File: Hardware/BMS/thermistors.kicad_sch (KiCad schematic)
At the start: 6 parts, among them U2 MAX14661ETI+T, U6 MAX14661ETI+T

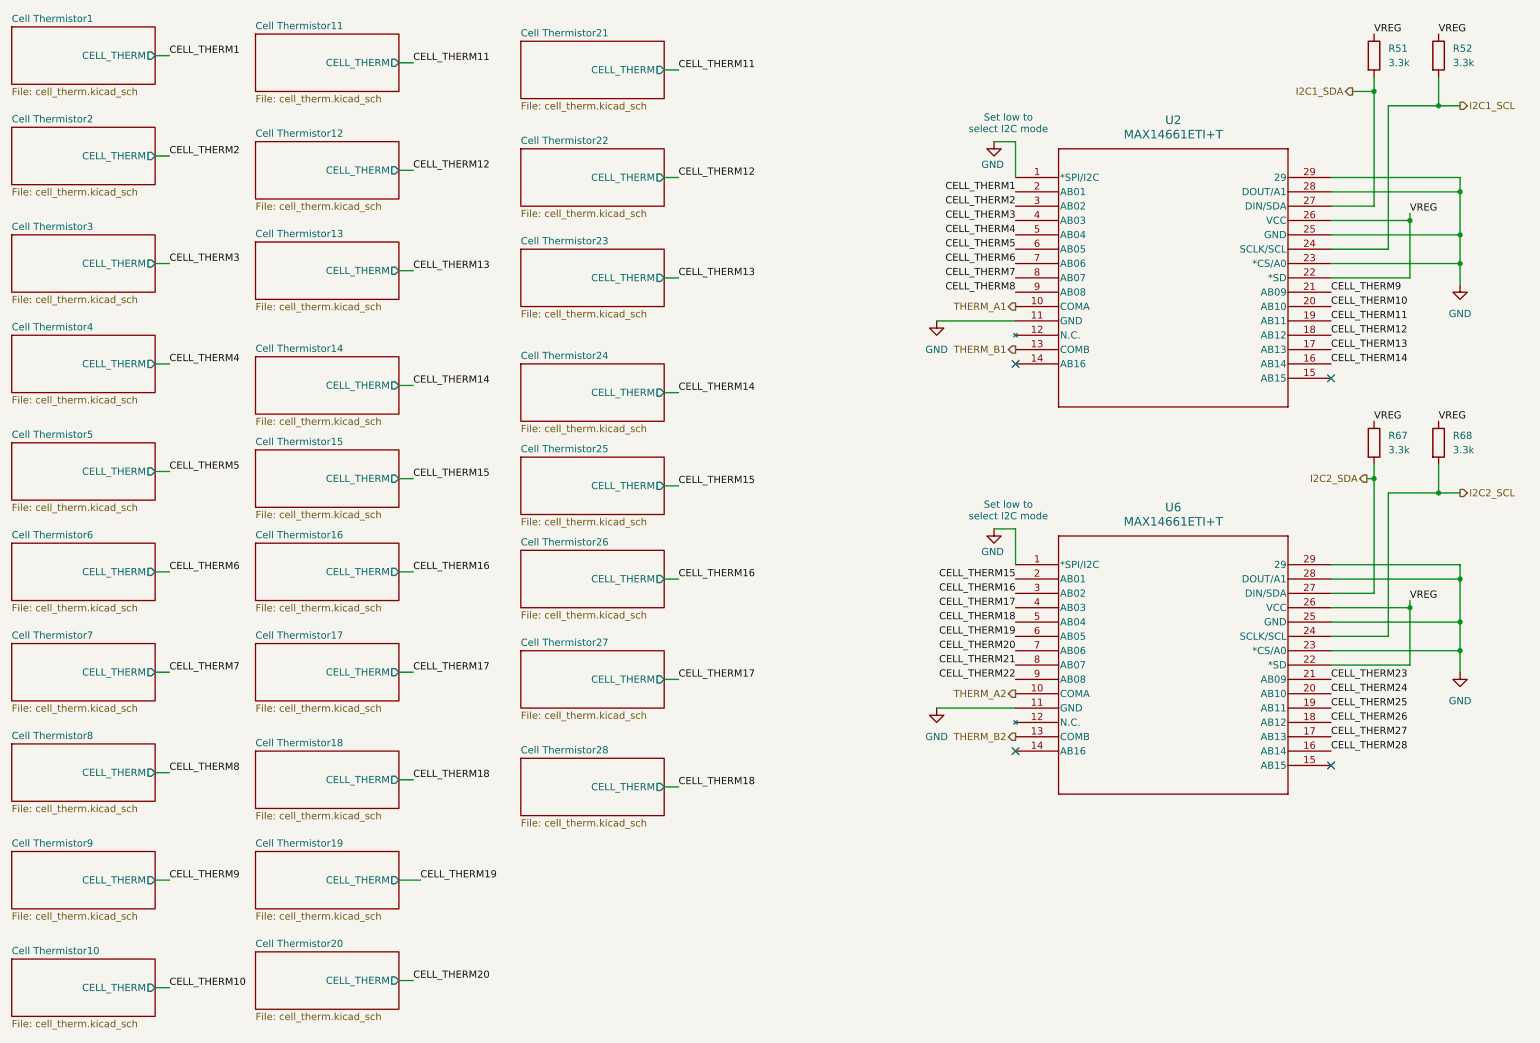
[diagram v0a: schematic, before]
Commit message: edits to the BMS
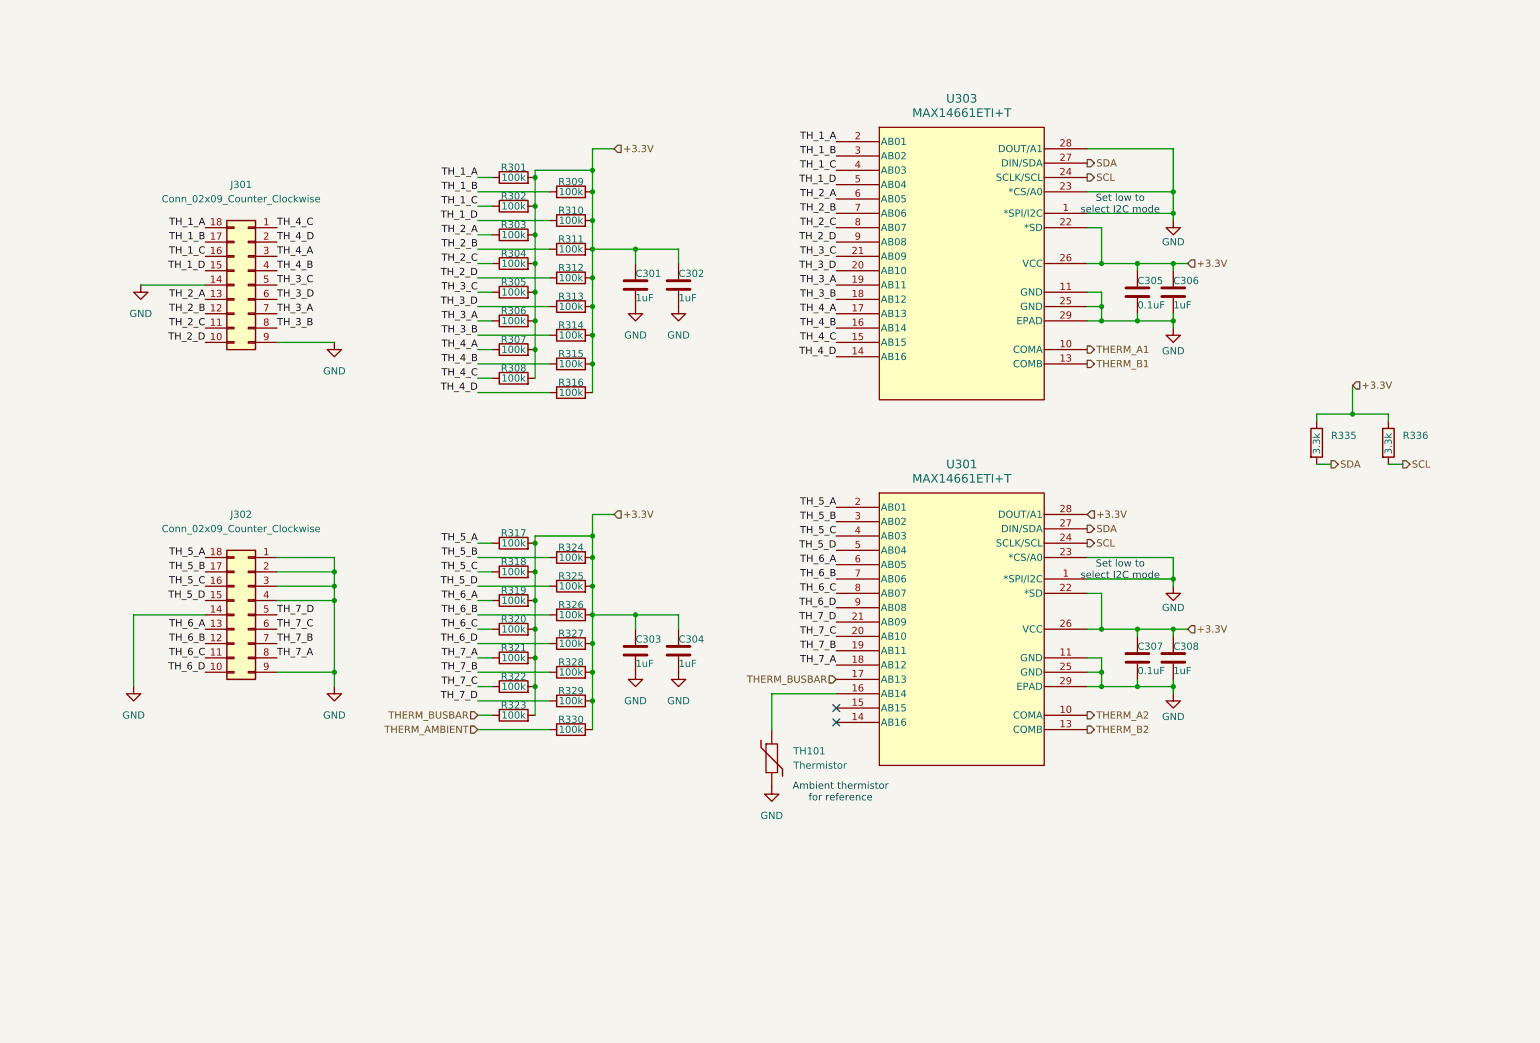
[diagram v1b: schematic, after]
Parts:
- removed R51, R52, R67, R68: 3.3k, symbol Device:R
- removed U2, U6: MAX14661ETI+T, 21-0139I_T2844-1_MXM, symbol MAX14661:MAX14661ETI+T
- added C301, C302, C303, C304, C306, C308: 1uF, Capacitor_SMD:C_0603_1608Metric, symbol Device:C
- added C305, C307: 0.1uF, Capacitor_SMD:C_0603_1608Metric, symbol Device:C
- added J301, J302: Conn_02x09_Counter_Clockwise, Connector_PinSocket_2.54mm:PinSocket_2x09_P2.54mm_Vertical, symbol Connector_Generic:Conn_02x09_Counter_Clockwise
- added R301, R302, R303, R304, R305, R306, R307, R308, R309, R310, R311, R312, R313, R314, R315, R316, R317, R318, R319, R320, R321, R322, R323, R324, R325, R326, R327, R328, R329, R330: 100k, symbol Device:R
- added R335, R336: 3.3k, symbol Device:R
- added TH101: Thermistor, Resistor_SMD:R_0603_1608Metric, symbol Device:Thermistor
- added U301, U303: MAX14661ETI+T, BAD_LIB:21-0139I_T2844-1_MXM, symbol OlinBAD:MAX14661ETI+T
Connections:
- net GND: now also C301.2, C302.2, C303.2, C304.2, C305.2, C306.2, C307.2, C308.2, J301.14 (Pin_14), J301.9 (Pin_9), J302.1 (Pin_1), J302.14 (Pin_14), J302.2 (Pin_2), J302.3 (Pin_3), J302.4 (Pin_4), J302.9 (Pin_9), TH101.2, U301.1 (*SPI/I2C), U301.11 (GND), U301.23 (*CS/A0), U301.25 (GND), U301.29 (EPAD), U303.1 (*SPI/I2C), U303.11 (GND), U303.23 (*CS/A0), U303.25 (GND), U303.28 (DOUT/A1), U303.29 (EPAD)
- net THERM_A1: now also U303.10 (COMA)
- net THERM_A2: now also U301.10 (COMA)
- net THERM_B1: now also U303.13 (COMB)
- net THERM_B2: now also U301.13 (COMB)
- new net: TH101.1, U301.16 (AB14)
- new net +3.3V: C301.1, C302.1, C303.1, C304.1, C305.1, C306.1, C307.1, C308.1, R301.2, R302.2, R303.2, R304.2, R305.2, R306.2, R307.2, R308.2, R309.2, R310.2, R311.2, R312.2, R313.2, R314.2, R315.2, R316.2, R317.2, R318.2, R319.2, R320.2, R321.2, R322.2, R323.2, R324.2, R325.2, R326.2, R327.2, R328.2, R329.2, R330.2, R335.1, R336.1, U301.22 (*SD), U301.26 (VCC), U301.28 (DOUT/A1), U303.22 (*SD), U303.26 (VCC)
- new net SCL: R336.2, U301.24 (SCLK/SCL), U303.24 (SCLK/SCL)
- new net SDA: R335.2, U301.27 (DIN/SDA), U303.27 (DIN/SDA)
- new net THERM_AMBIENT: R330.1
- new net THERM_BUSBAR: R323.1, U301.17 (AB13)
- new net TH_1_A: J301.18 (Pin_18), R301.1, U303.2 (AB01)
- new net TH_1_B: J301.17 (Pin_17), R309.1, U303.3 (AB02)
- new net TH_1_C: J301.16 (Pin_16), R302.1, U303.4 (AB03)
- new net TH_1_D: J301.15 (Pin_15), R310.1, U303.5 (AB04)
- new net TH_2_A: J301.13 (Pin_13), R303.1, U303.6 (AB05)
- new net TH_2_B: J301.12 (Pin_12), R311.1, U303.7 (AB06)
- new net TH_2_C: J301.11 (Pin_11), R304.1, U303.8 (AB07)
- new net TH_2_D: J301.10 (Pin_10), R312.1, U303.9 (AB08)
- new net TH_3_A: J301.7 (Pin_7), R306.1, U303.19 (AB11)
- new net TH_3_B: J301.8 (Pin_8), R314.1, U303.18 (AB12)
- new net TH_3_C: J301.5 (Pin_5), R305.1, U303.21 (AB09)
- new net TH_3_D: J301.6 (Pin_6), R313.1, U303.20 (AB10)
- new net TH_4_A: J301.3 (Pin_3), R307.1, U303.17 (AB13)
- new net TH_4_B: J301.4 (Pin_4), R315.1, U303.16 (AB14)
- new net TH_4_C: J301.1 (Pin_1), R308.1, U303.15 (AB15)
- new net TH_4_D: J301.2 (Pin_2), R316.1, U303.14 (AB16)
- new net TH_5_A: J302.18 (Pin_18), R317.1, U301.2 (AB01)
- new net TH_5_B: J302.17 (Pin_17), R324.1, U301.3 (AB02)
- new net TH_5_C: J302.16 (Pin_16), R318.1, U301.4 (AB03)
- new net TH_5_D: J302.15 (Pin_15), R325.1, U301.5 (AB04)
- new net TH_6_A: J302.13 (Pin_13), R319.1, U301.6 (AB05)
- new net TH_6_B: J302.12 (Pin_12), R326.1, U301.7 (AB06)
- new net TH_6_C: J302.11 (Pin_11), R320.1, U301.8 (AB07)
- new net TH_6_D: J302.10 (Pin_10), R327.1, U301.9 (AB08)
- new net TH_7_A: J302.8 (Pin_8), R321.1, U301.18 (AB12)
- new net TH_7_B: J302.7 (Pin_7), R328.1, U301.19 (AB11)
- new net TH_7_C: J302.6 (Pin_6), R322.1, U301.20 (AB10)
- new net TH_7_D: J302.5 (Pin_5), R329.1, U301.21 (AB09)
- no-connect marks 4 -> 2
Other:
- removed sheet Cell Thermistor1
- removed sheet Cell Thermistor10
- removed sheet Cell Thermistor11
- removed sheet Cell Thermistor12
- removed sheet Cell Thermistor13
- removed sheet Cell Thermistor14
- removed sheet Cell Thermistor15
- removed sheet Cell Thermistor16
- removed sheet Cell Thermistor17
- removed sheet Cell Thermistor18
- removed sheet Cell Thermistor19
- removed sheet Cell Thermistor2
- removed sheet Cell Thermistor20
- removed sheet Cell Thermistor21
- removed sheet Cell Thermistor22
- removed sheet Cell Thermistor23
- removed sheet Cell Thermistor24
- removed sheet Cell Thermistor25
- removed sheet Cell Thermistor26
- removed sheet Cell Thermistor27
- removed sheet Cell Thermistor28
- removed sheet Cell Thermistor3
- removed sheet Cell Thermistor4
- removed sheet Cell Thermistor5
- removed sheet Cell Thermistor6
- removed sheet Cell Thermistor7
- removed sheet Cell Thermistor8
- removed sheet Cell Thermistor9
- note added: "Ambient thermistor for reference"
